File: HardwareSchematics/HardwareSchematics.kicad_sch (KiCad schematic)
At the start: 2 parts, among them U1 ESP32-WROOM-32, U2 MPU-6050

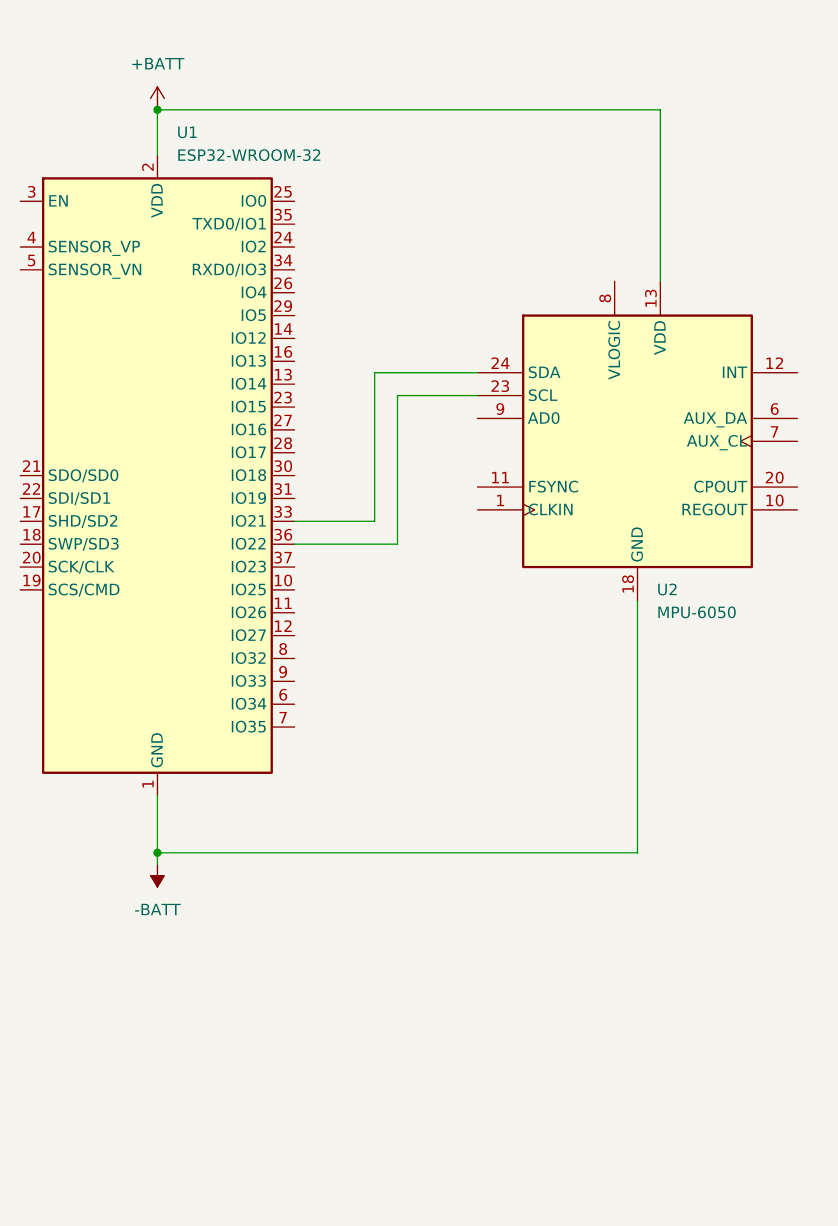
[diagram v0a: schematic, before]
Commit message: update schematics
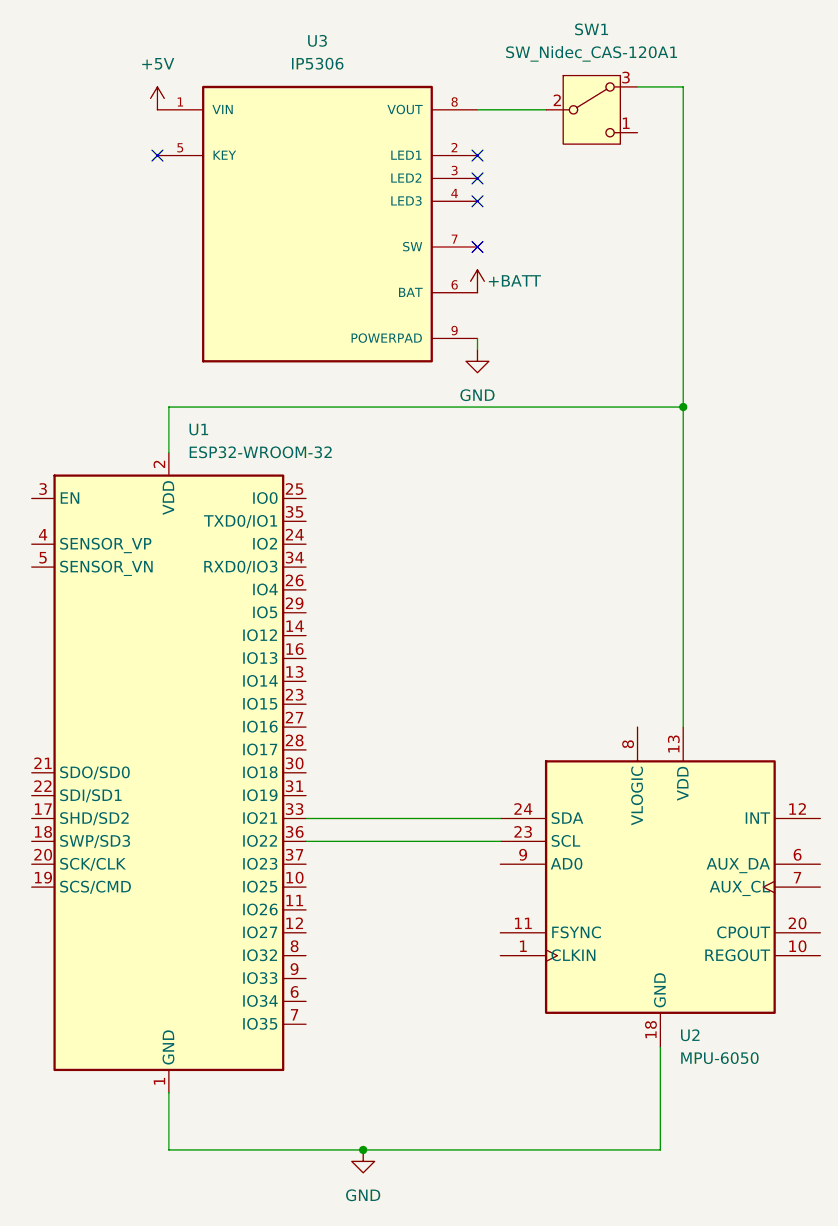
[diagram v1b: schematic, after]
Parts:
- added SW1: SW_Nidec_CAS-120A1, Button_Switch_SMD:Nidec_Copal_CAS-120A, symbol Switch:SW_Nidec_CAS-120A1
- added U3: IP5306, IP5306:SOP127P600X165-9N, symbol IP5306:IP5306
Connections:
- net +BATT: now also U3.6 (BAT); no longer U1.2 (VDD), U2.13 (VDD)
- net -BATT renamed GND
- net GND: now also U3.9 (POWERPAD)
- new net: SW1.2 (B), U3.8 (VOUT)
- new net: SW1.3 (A), U1.2 (VDD), U2.13 (VDD)
- new net +5V: U3.1 (VIN)
- no-connect marks 0 -> 5
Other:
- moved on the sheet: U1, U2
